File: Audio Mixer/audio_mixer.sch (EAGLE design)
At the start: 67 parts, among them IC1 OPA2134P

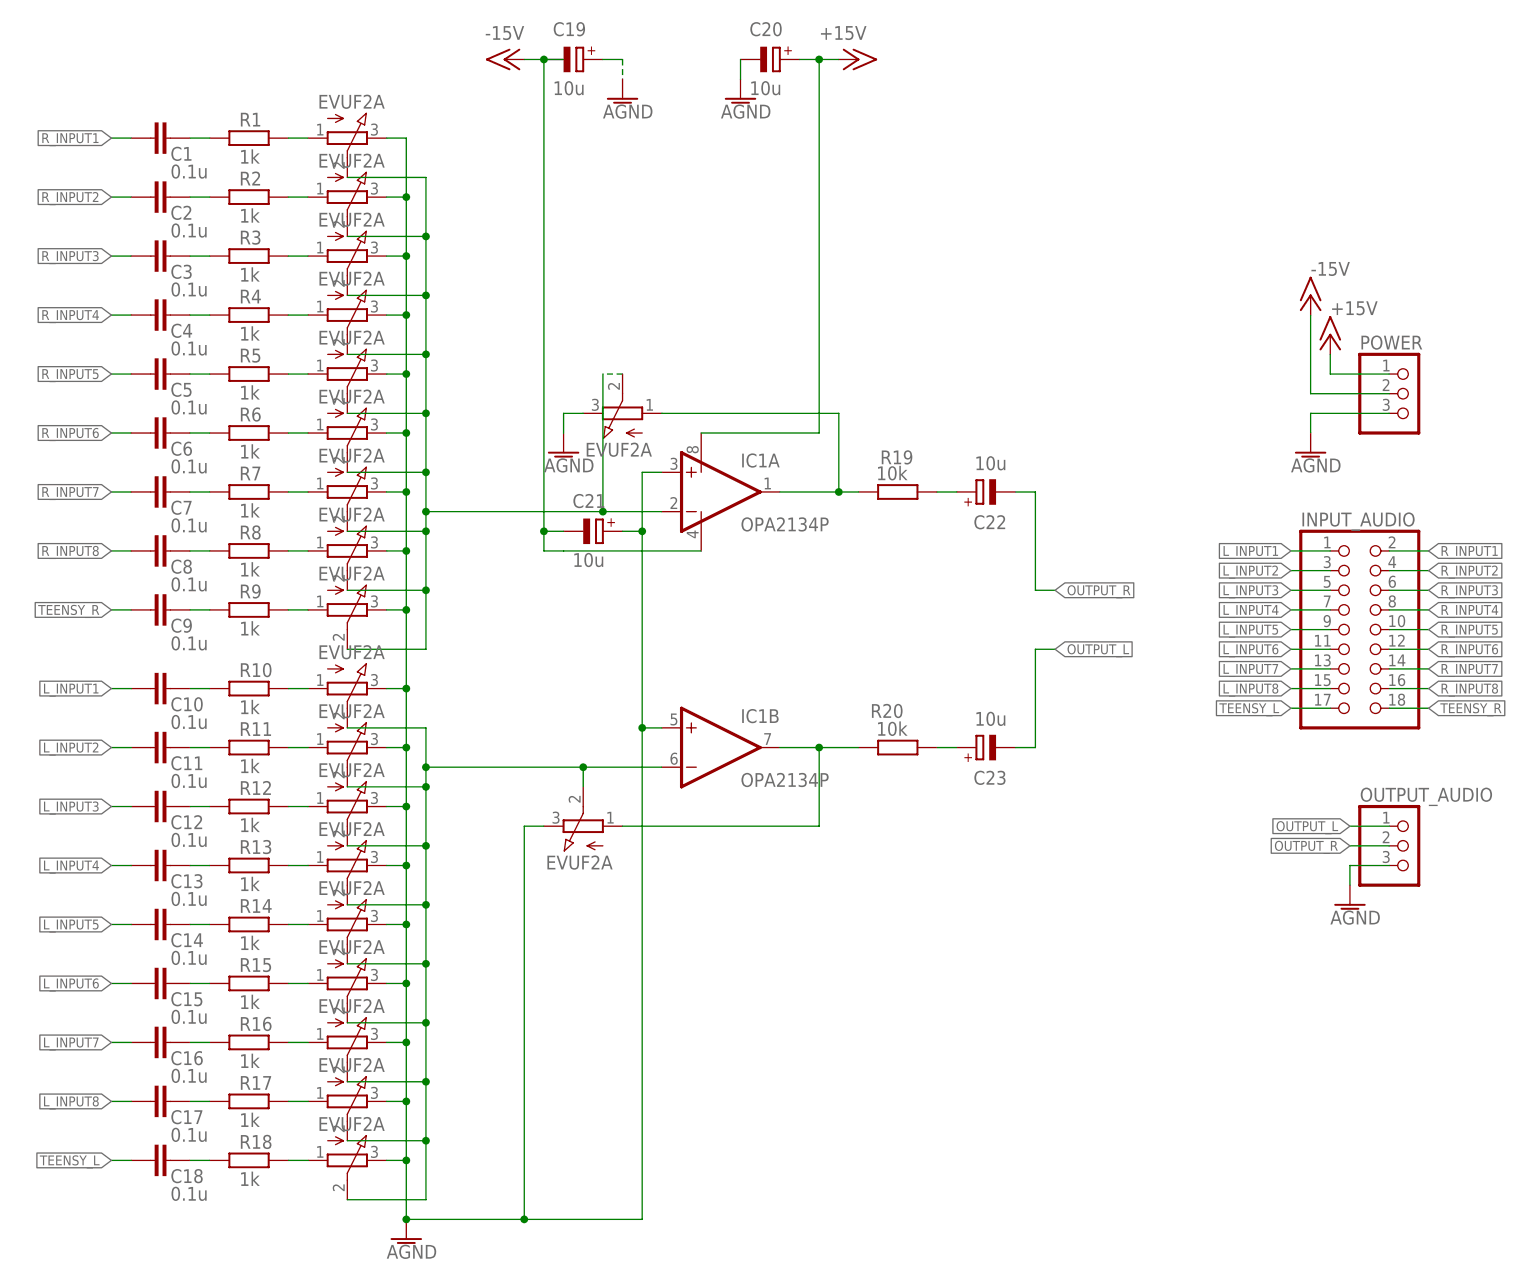
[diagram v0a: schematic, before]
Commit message: old seperate files
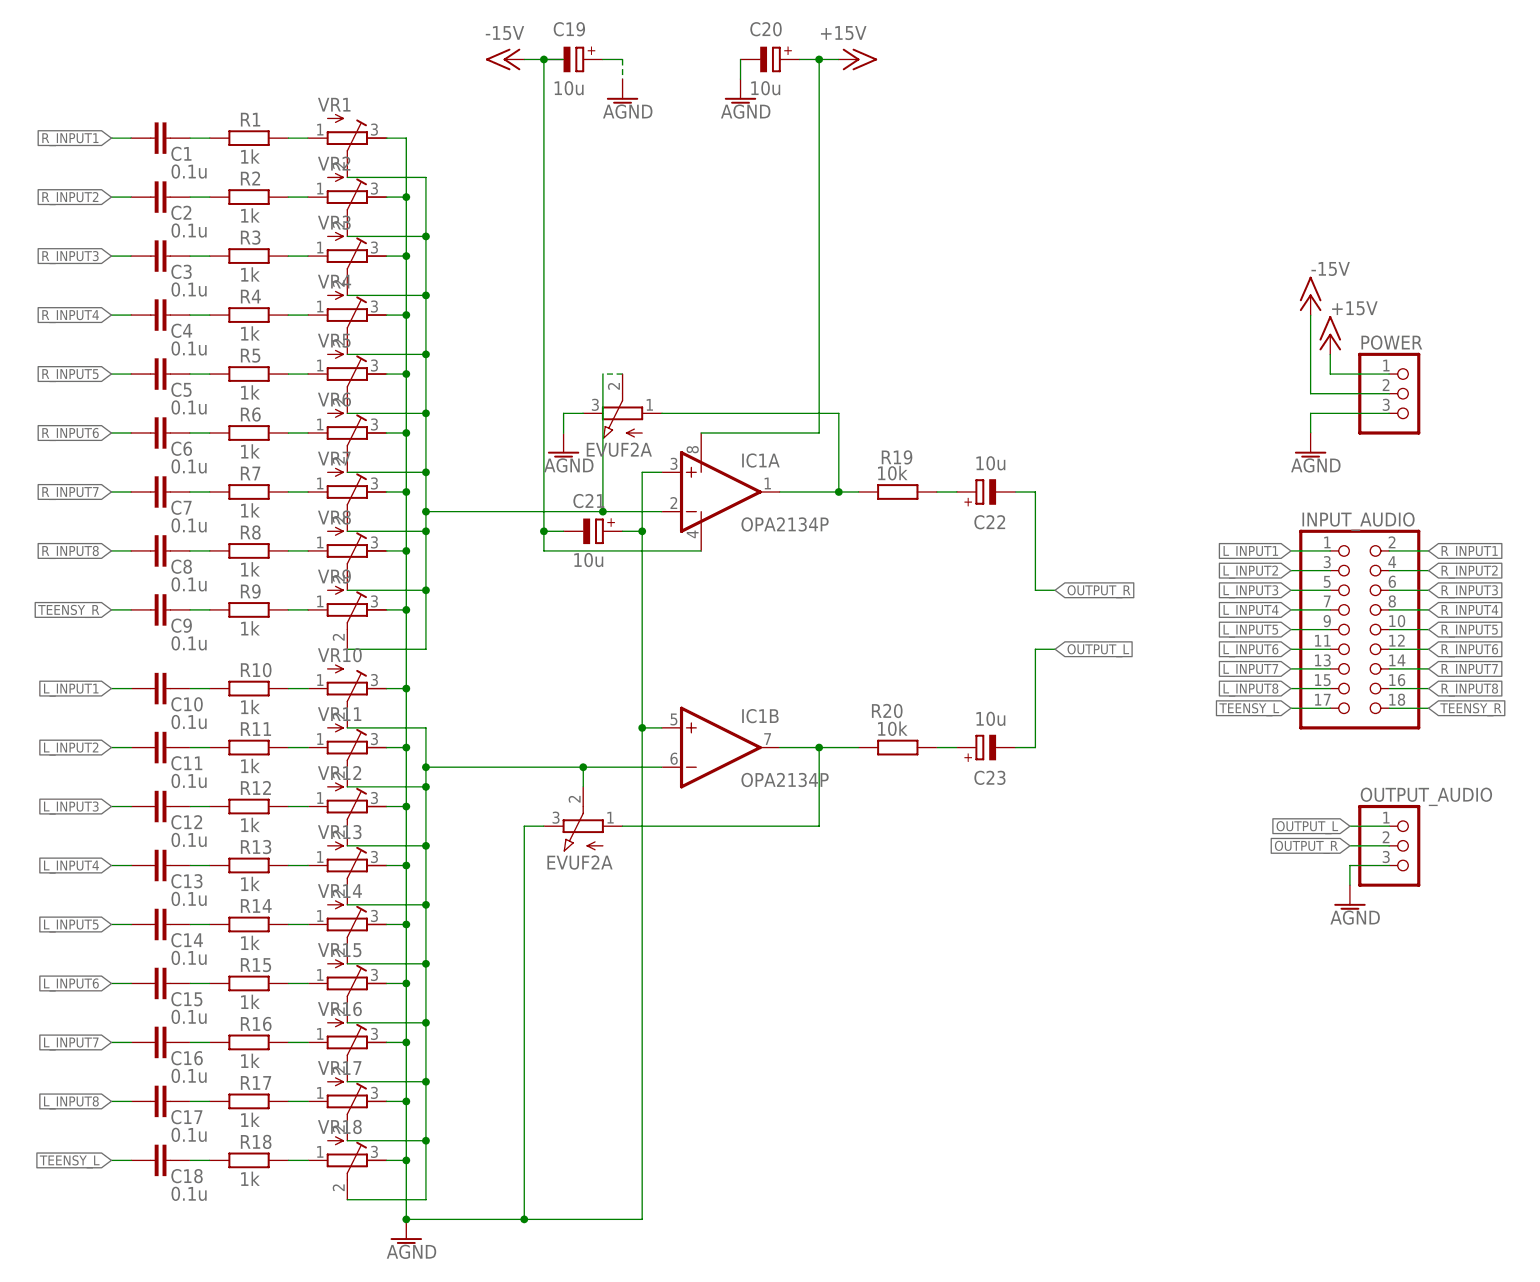
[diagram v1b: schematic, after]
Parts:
- VR1, VR10, VR11, VR12, VR13, VR14, VR15, VR16, VR17, VR18, VR2, VR3, VR4, VR5, VR6, VR7, VR8, VR9: value EVUF2A -> (none); device pot:EVUF2A -> rcl:R-TRIMM3339P
